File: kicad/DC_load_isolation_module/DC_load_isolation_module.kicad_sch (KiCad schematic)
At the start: 60 parts, among them J6 USB_B, Q1 MMBT5401, Q13 AO3400A, Q5 MMBT5401, Q6 MMBT5551L, U14 AMS1117-3.3, U17 CH340C, U18 TL431DBZ, U2 MC34063AD

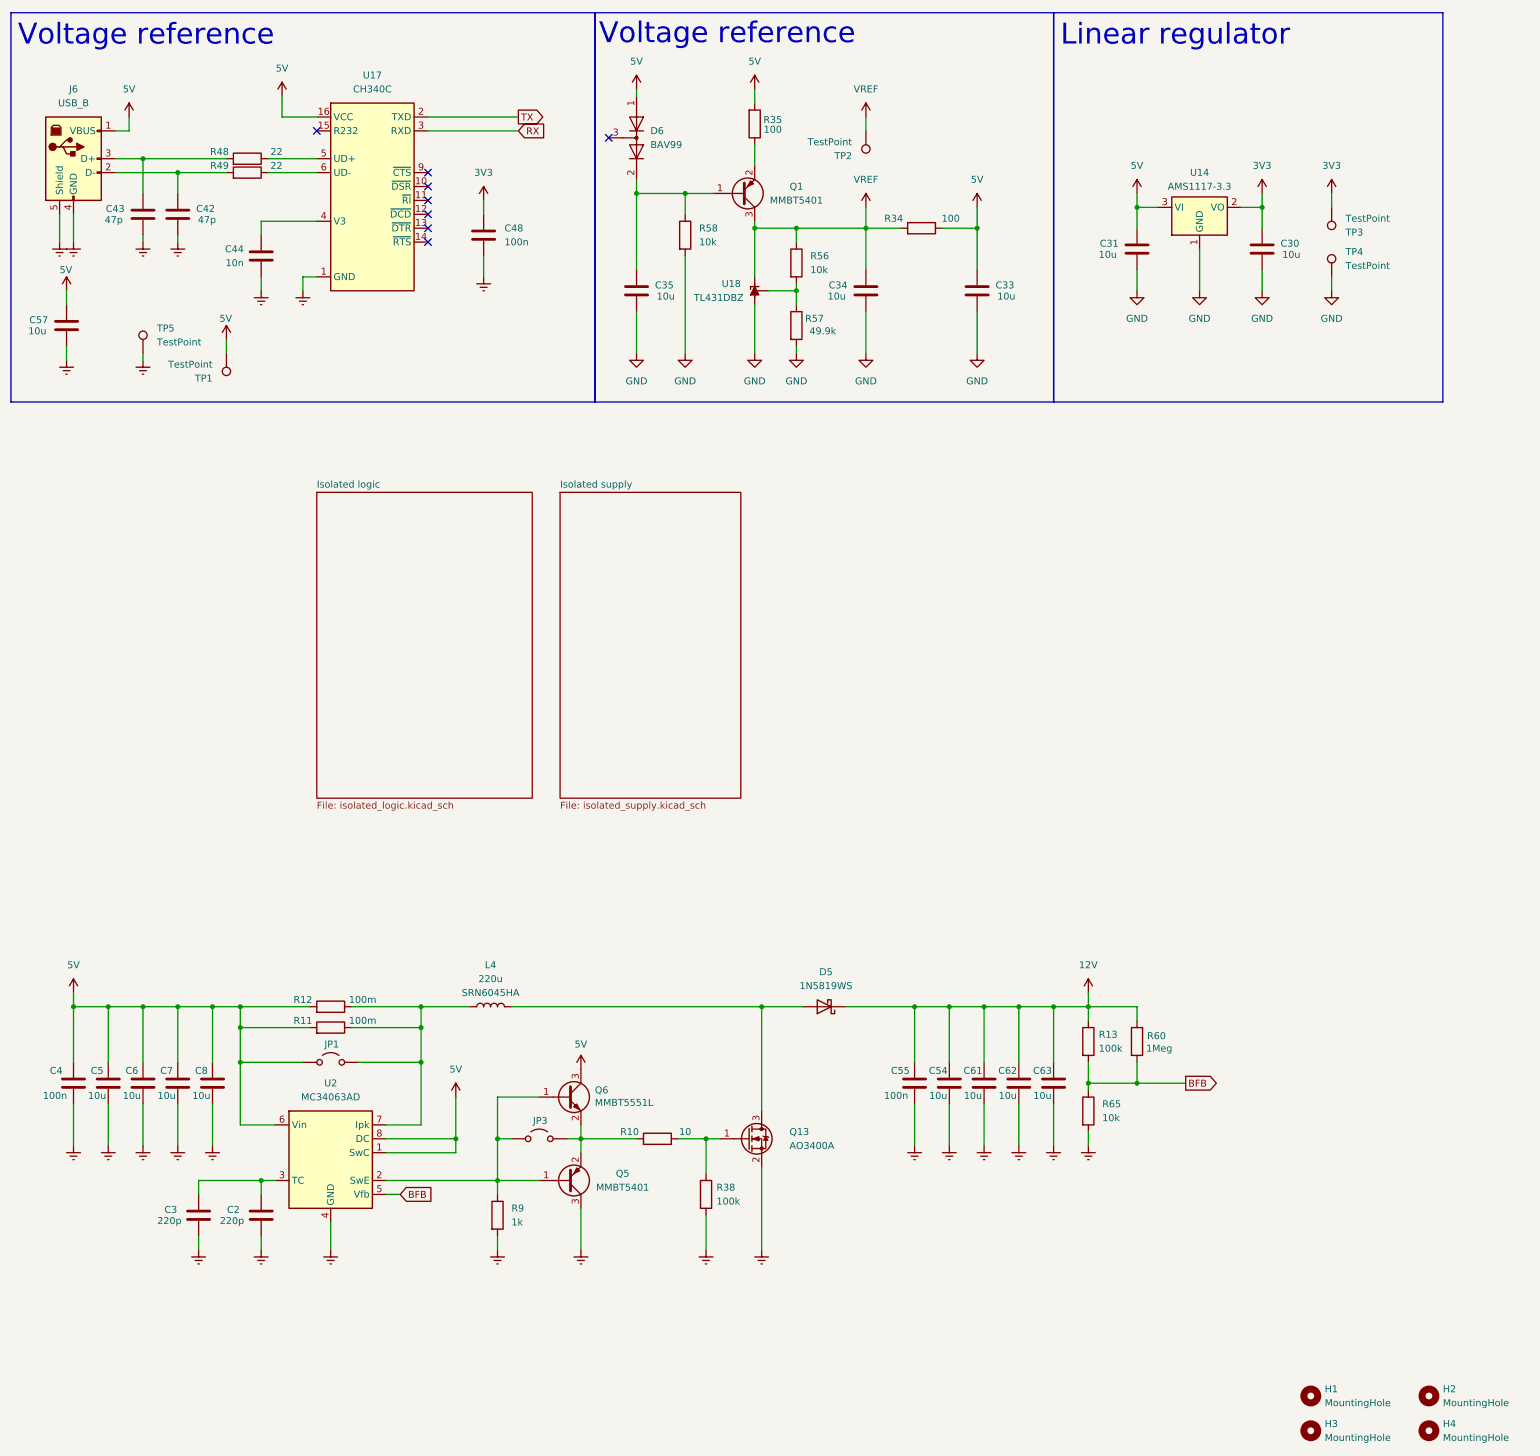
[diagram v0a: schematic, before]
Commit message: Idk.
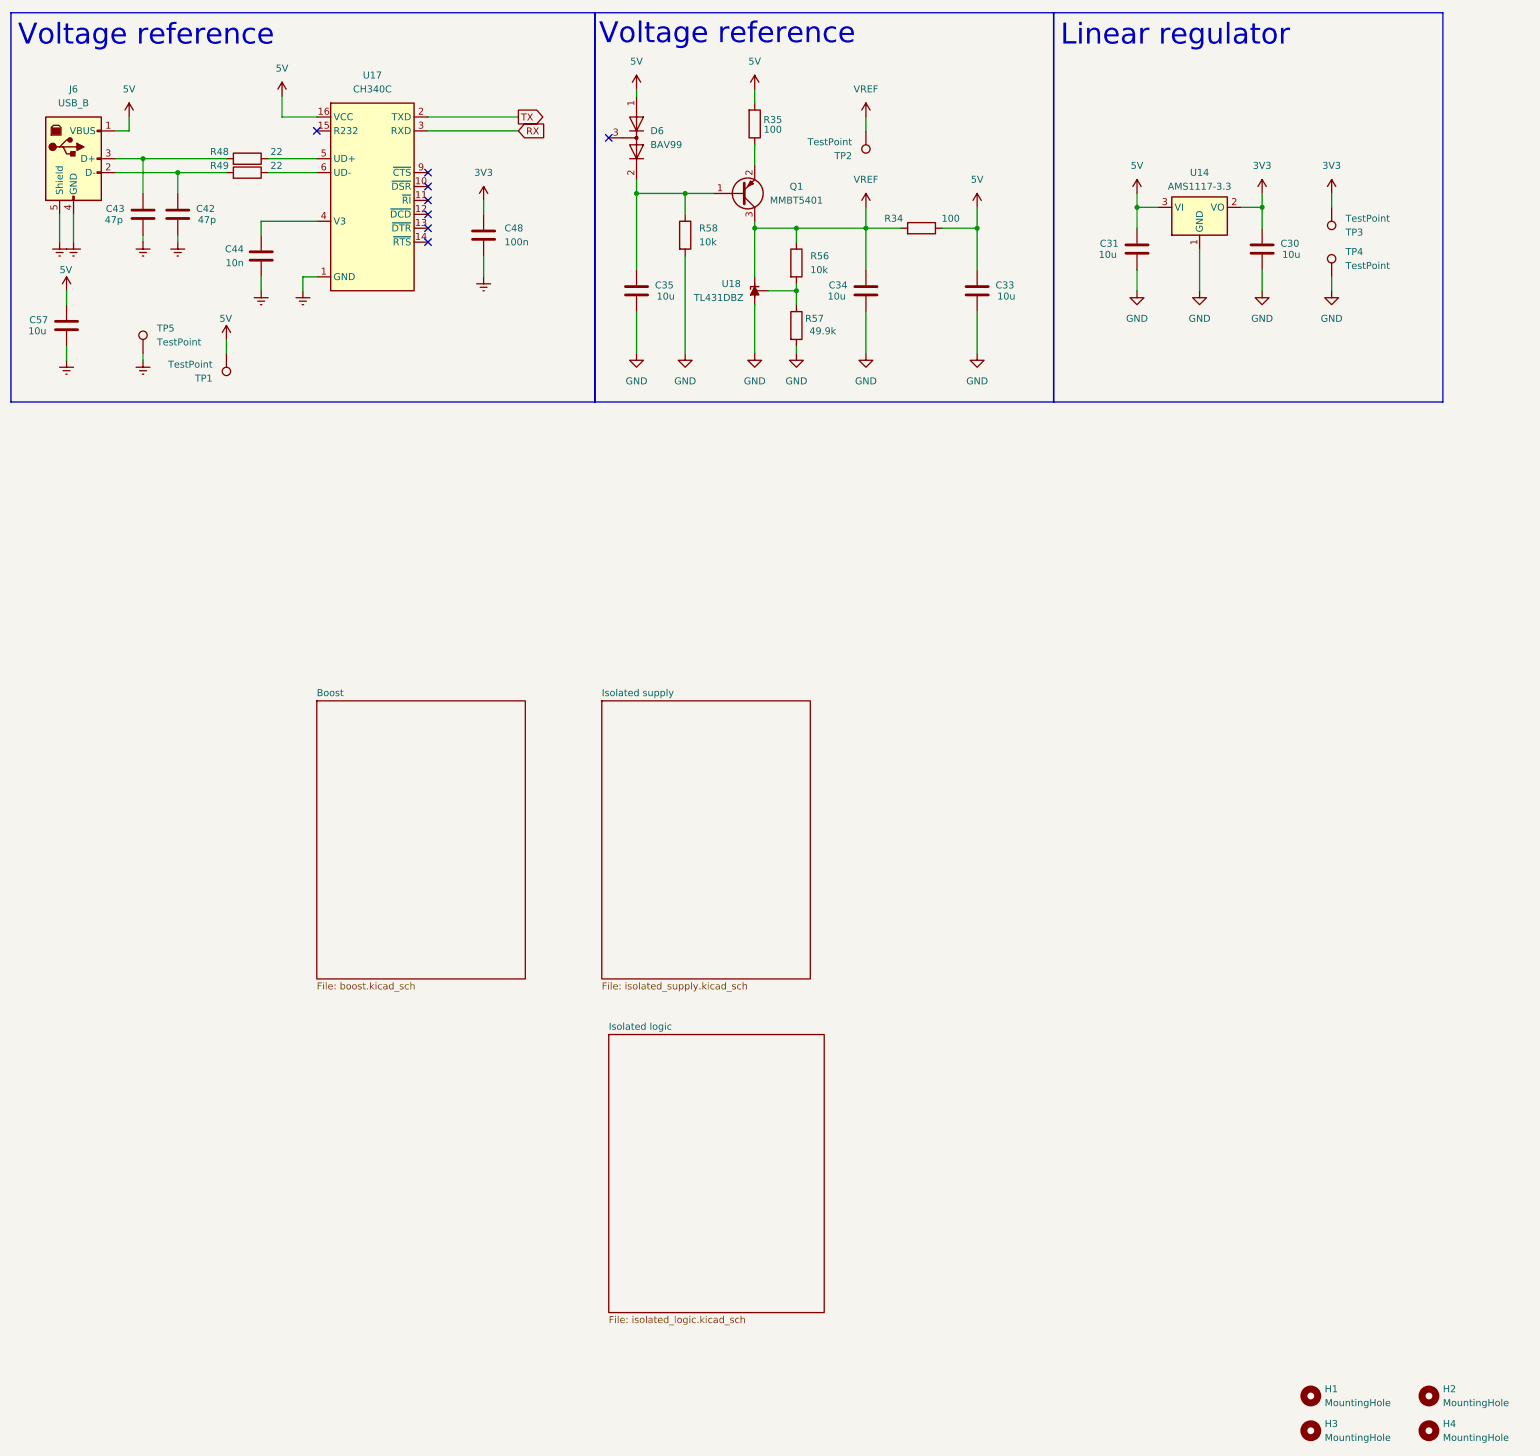
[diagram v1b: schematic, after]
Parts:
- removed C2, C3: 220p, Capacitor_SMD:C_0603_1608Metric_Pad1.08x0.95mm_HandSolder, symbol Device:C
- removed C4, C55: 100n, Capacitor_SMD:C_0603_1608Metric_Pad1.08x0.95mm_HandSolder, symbol Device:C
- removed C5, C54, C6, C61, C62, C63, C7, C8: 10u, Capacitor_SMD:C_0603_1608Metric_Pad1.08x0.95mm_HandSolder, symbol Device:C
- removed D5: 1N5819WS, Diode_SMD:D_SOD-323, symbol Diode:1N5819WS
- removed JP1, JP3: Jumper_2_Open, Jumper:SolderJumper-2_P1.3mm_Open_RoundedPad1.0x1.5mm, symbol Jumper:Jumper_2_Open
- removed L4: 220u, DC_load:L_Bourns_SRN6045TA, symbol solar_push_pull_sym_lib:SRN6045HA-4R7Y
- removed Q13: AO3400A, Package_TO_SOT_SMD:SOT-23, symbol Transistor_FET:AO3400A
- removed Q5: MMBT5401, Package_TO_SOT_SMD:SOT-23, symbol Transistor_BJT:MMBT3906
- removed Q6: MMBT5551L, Package_TO_SOT_SMD:SOT-23, symbol Transistor_BJT:MMBT5551L
- removed R10: 10, Resistor_SMD:R_0603_1608Metric_Pad0.98x0.95mm_HandSolder, symbol Device:R
- removed R11, R12: 100m, Resistor_SMD:R_1206_3216Metric_Pad1.30x1.75mm_HandSolder, symbol Device:R
- removed R13, R38: 100k, Resistor_SMD:R_0603_1608Metric_Pad0.98x0.95mm_HandSolder, symbol Device:R
- removed R60: 1Meg, Resistor_SMD:R_0603_1608Metric_Pad0.98x0.95mm_HandSolder, symbol Device:R
- removed R65: 10k, Resistor_SMD:R_0603_1608Metric_Pad0.98x0.95mm_HandSolder, symbol Device:R
- removed R9: 1k, Resistor_SMD:R_0603_1608Metric_Pad0.98x0.95mm_HandSolder, symbol Device:R
- removed U2: MC34063AD, Package_SO:SOIC-8_3.9x4.9mm_P1.27mm, symbol Regulator_Switching:MC34063AD
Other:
- added sheet Boost (boost.kicad_sch)
